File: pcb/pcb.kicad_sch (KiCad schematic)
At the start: 29 parts, among them U1 1117-3.3, U2 NORTH, U3 SOUTH, U4 EAST, U5 WEST, U6 RP2040

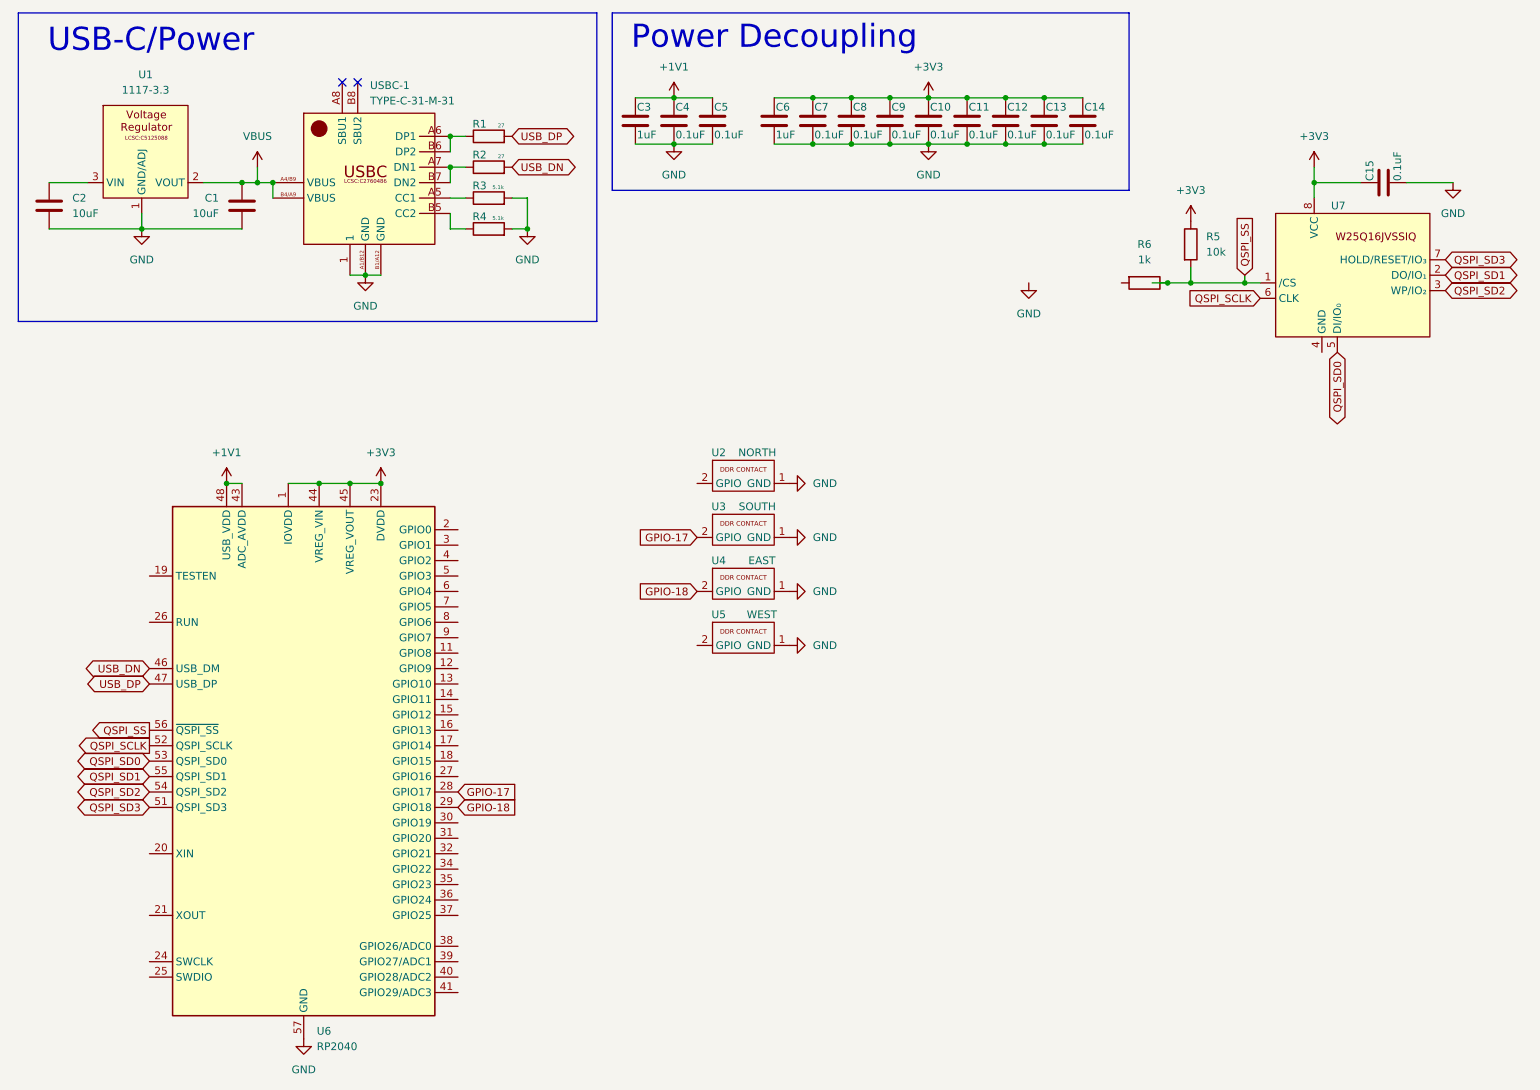
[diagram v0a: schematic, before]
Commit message: work on schematic
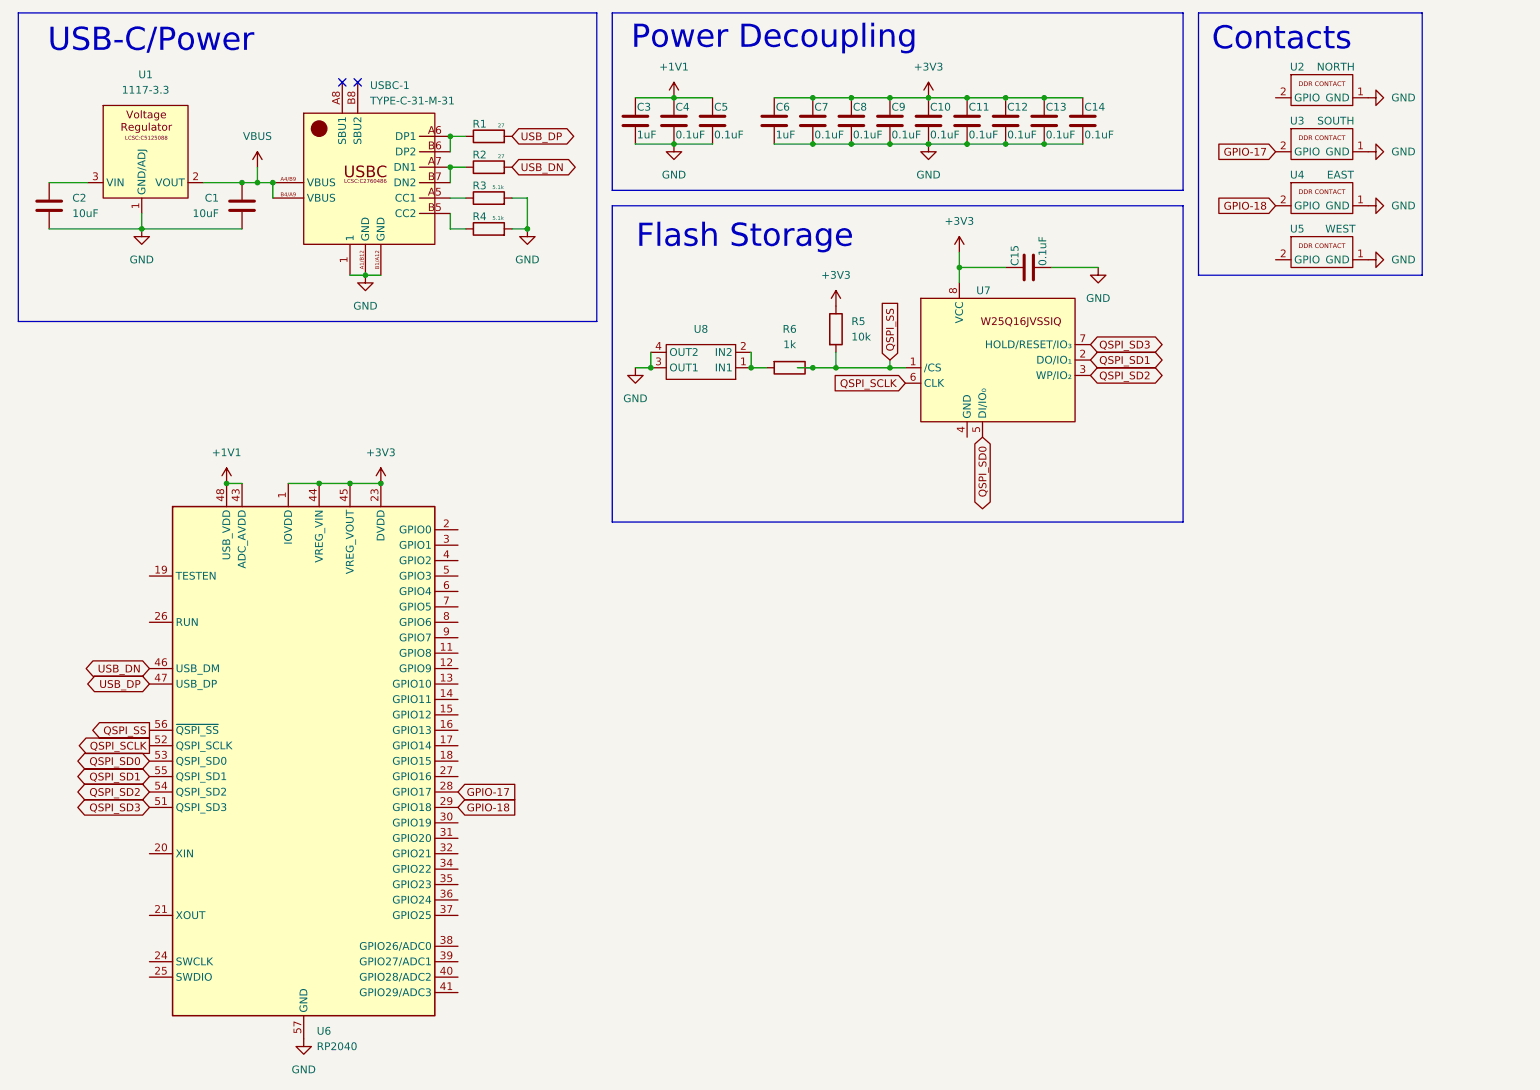
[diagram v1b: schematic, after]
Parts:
- added U8: (no value), Andrews_Library:LCSC_TS-1089S-02526_C455282, symbol Andrews_Library:LCSC_TS-1089S-02526_C455282
- U7: footprint (none) -> Andrews_Library:LCSC_W25Q16JVSSIQ_C131025
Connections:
- net GND: now also U8.3 (OUT1), U8.4 (OUT2)
- net at R6.2: now also U8.1 (IN1), U8.2 (IN2)
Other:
- note added: "Contacts"
- note added: "Flash Storage"
- moved on the sheet: C15, R5, R6, U2, U3, U4, U5, U7
